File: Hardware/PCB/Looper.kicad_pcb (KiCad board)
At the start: 2 copper layers, 78.5 x 110.1 mm, 69 parts, among them J1 Out right, J11 Conn_01x05, J12 Conn_01x05, J2 In left, J3 Trig Loop, J4 Out left, J5 In right, J6 Eurorack_Power, J7 Conn_01x05, J8 Conn_01x05, Q1 MMBT3904, U1 TL074, U2 TL074

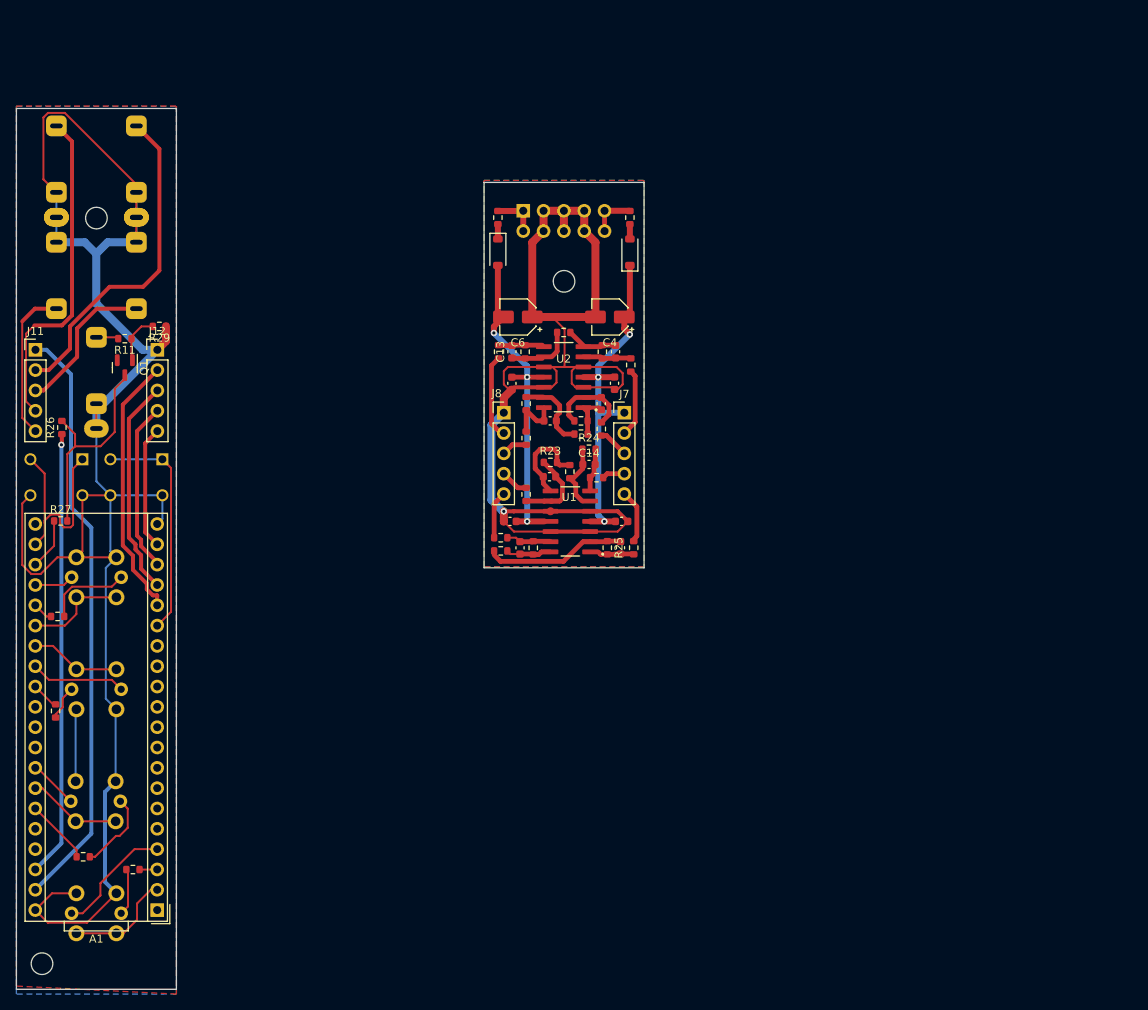
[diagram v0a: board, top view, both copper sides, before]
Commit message: Version 1.0d hardware
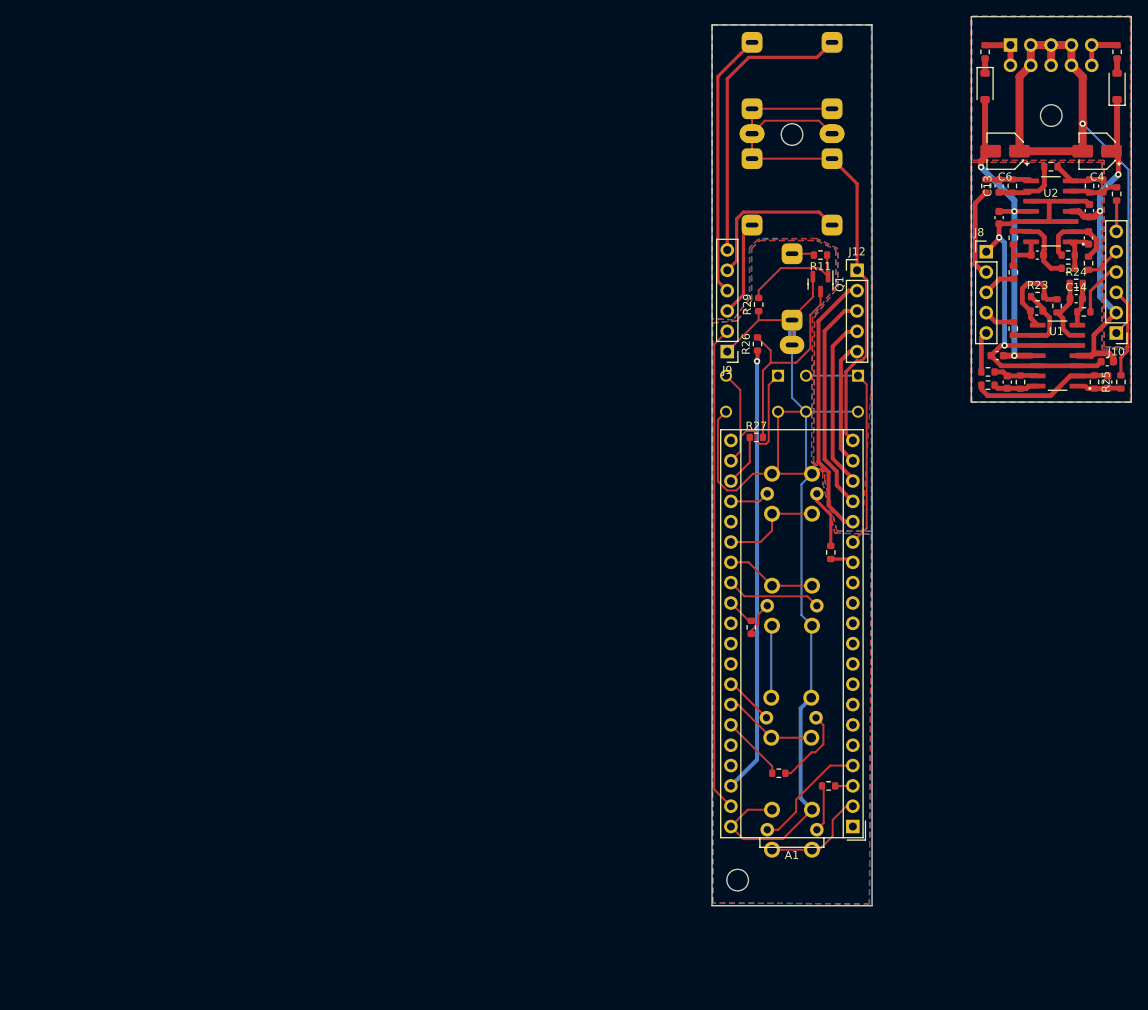
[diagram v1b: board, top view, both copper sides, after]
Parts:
- removed J11, J7: Conn_01x05, Connector_PinHeader_2.54mm:PinHeader_1x05_P2.54mm_Vertical
- added J10: Conn_01x06_Socket, Connector_PinHeader_2.54mm:PinHeader_1x06_P2.54mm_Vertical, F.Cu at (206.5, 86.1)
- added J9: Conn_01x06_Pin, Connector_PinHeader_2.54mm:PinHeader_1x06_P2.54mm_Vertical, F.Cu at (157.9, 88.4)
- moved R3 97.0 mm to (170.8, 113.5), turned to -90 degrees
- moved J12 88.0 mm to (174.1, 78.3)
- moved MOUNT1 87.6 mm to (159.2, 154.5)
- moved Q1 87.6 mm to (169.5, 80.0)
- moved R1 87.6 mm to (164.3, 141.1)
- moved R11 87.6 mm to (169.5, 76.4)
- moved R26 87.6 mm to (161.7, 87.5)
- moved J1 87.6 mm to (161.0, 67.7)
- moved J2 87.6 mm to (171.0, 54.7)
- moved J3 87.6 mm to (166.0, 81.1)
- moved J4 87.6 mm to (161.0, 54.7)
- moved J5 87.6 mm to (171.0, 67.7)
- moved MOUNT1 87.6 mm to (166.0, 61.3)
- moved R2 87.6 mm to (160.9, 122.9)
- moved R4 87.6 mm to (170.5, 142.7)
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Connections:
- A1 pad 14: unconnected-(A1-USART1_TX-Pad14) -> SWITCH_1_RED
- A1 pad 20: GND -> AGND
- A1 pad 25: SWITCH_1_RED -> unconnected-(A1-ADC_INP7-Pad25)
- C1 pad 1: GND -> AGND
- C11 pad 2: GND -> AGND
- C12 pad 1: GND -> AGND
- C5 pad 2: GND -> AGND
- J1 pad S: GND -> AGND
- J1 pad TN: GND -> AGND
- J12 pad 1: GND -> AGND
- J2 pad S: GND -> AGND
- J2 pad TN: GND -> AGND
- J4 pad S: GND -> AGND
- J4 pad TN: GND -> AGND
- J5 pad S: GND -> AGND
- J5 pad TN: GND -> AGND
- J8 pad 1: GND -> AGND
- U1 pad 10: GND -> AGND
- U1 pad 12: GND -> AGND
- U1 pad 3: GND -> AGND
- U1 pad 5: GND -> AGND
- U2 pad 10: GND -> AGND
- U2 pad 12: GND -> AGND
- U2 pad 3: GND -> AGND
- U2 pad 5: GND -> AGND
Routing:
- net GND: track 365.9 -> 223.9 mm
- net AGND: track 0.00 -> 138.3 mm, vias 0 -> 2
- net +12V: track 119.0 -> 105.8 mm, vias 3 -> 2
- net In Left: track 50.0 -> 40.2 mm
- net Net-(Q1-B): track 6.03 -> 13.8 mm
- net Out Left: track 44.1 -> 40.1 mm
- net Net-(R3-Pad1): track 10.8 -> 7.24 mm
- net Out Right: track 25.8 -> 23.3 mm
- net In Right: track 22.7 -> 24.3 mm
- net DAISY_AUDIO_IN_R: track 30.4 -> 31.8 mm
- net DAISY_AUDIO_IN_L: track 43.5 -> 44.7 mm
- net DAISY_AUDIO_OUT_L: track 24.6 -> 25.3 mm
- net DAISY_AUDIO_OUT_R: track 21.4 -> 20.8 mm
- net Net-(C3-Pad2): track 7.09 -> 6.59 mm
- added copper zone on B.Cu, net AGND
- added copper zone on F.Cu, net AGND
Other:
- board size 78.5 x 110.1 mm -> 52.4 x 111.1 mm
- board text added: "Loop v1.0d"
- board text removed: "Loop v1.0c"
